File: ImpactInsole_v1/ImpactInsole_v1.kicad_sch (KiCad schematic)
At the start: 0 parts

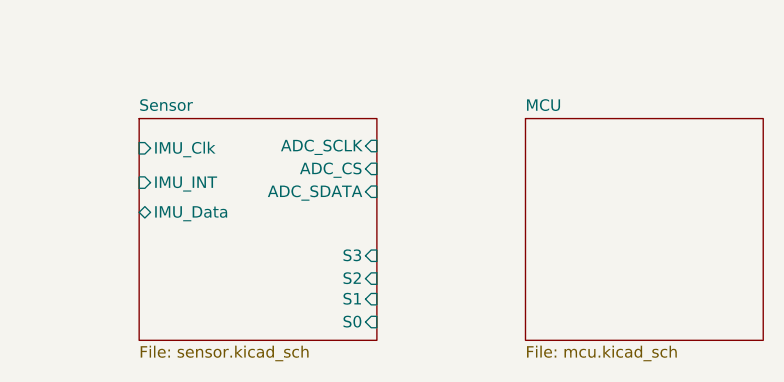
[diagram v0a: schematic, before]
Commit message: pcb begnnings + more libs
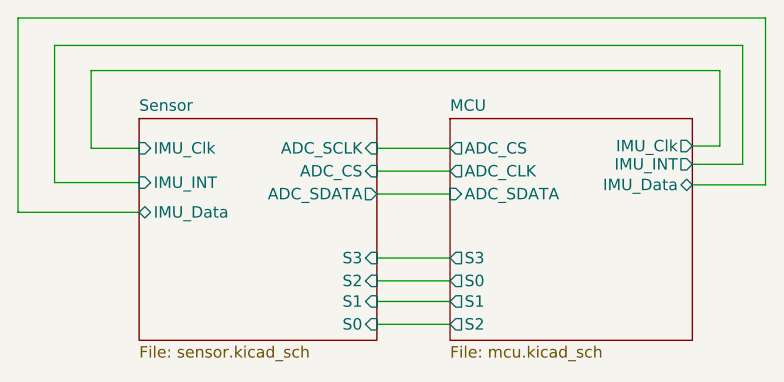
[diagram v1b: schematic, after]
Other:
- sheet MCU ports: added ADC_CLK, ADC_CS, ADC_SDATA, IMU_Clk, IMU_Data, IMU_INT, S0, S1, S2, S3; removed none
